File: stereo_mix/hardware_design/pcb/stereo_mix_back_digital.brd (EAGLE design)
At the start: 75 x 100 mm, 233 parts, among them IC1 TL072D, IC10 LD117AS50TR, IC11 MCP4822E-SN, IC12 MCP4822E-SN, IC13 MCP4822E-SN, IC14 MCP4822E-SN, IC15 TL072D, IC16 TL072D, IC17 TL072D, IC18 TL072D, IC2 TL072D, IC3 TL072D, IC4 TL072D, IC5 TL072D, IC6 TL072D, IC7 TL072D, IC8 TL072D, IC9 TL072D, Q1 20MHz, U1 MCP6002_, U10 MCP6002_, U11 MCP4922, U12 MCP4922, U13 ATMEGA328P-AU, U14 TEXAS_INSTRUMENTS_LM4040C5IDB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, U15 TEXAS_INSTRUMENTS_LM4040C10ID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, U16 TEXAS_INSTRUMENTS_LM4040C10ID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, U2 MCP6002_, U3 MCP6002_, U4 MCP6002_, U5 MCP4922, U6 MCP4922, U7 MCP6002_, U8 MCP6002_, U9 MCP6002_

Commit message: Add new revision of stereo_mix_back hardware, and associated assembly files
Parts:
- removed IC10: LD117AS50TR, v-reg:SOT223
- removed IC11, IC12, IC13, IC14: MCP4822E-SN, dac:SOIC-8
- removed IC15, IC16, IC17, IC18, IC2, IC3, IC4, IC5, IC6, IC7, IC8, IC9: TL072D, linear:SO08
- added D3: LM4040AIM3-5.0, jhbruhn-ref:SOT23
- added D4, D5: LM4040AIM3-10.0, jhbruhn-ref:SOT23
- added U17, U18, U21, U22, U26, U27, U28, U29, U30: TL072AD, jhbruhn-opamp:SOIC8
- added U19, U20, U24, U25: MCP4822E-SN, jhbruhn-dac:SOIC8
- added U23: ATMEGA328P-AU, jhbruhn-mcu:TQFP-32
- C1, C10, C13, C14, C15, C16, C17, C18, C2, C21, C22, C23, C24, C27, C28, C29, C3, C30, C31, C32, C36, C37, C38, C4, C47, C5, C50, C51, C52, C53, C54, C58, C6, C61, C62, C63, C7, C8, C9: device resistor:C0402 -> jhbruhn-cr:C0402
- C11, C12, C19, C20: value 100nF -> 4.7nF; device resistor:C0402 -> jhbruhn-cr:C0402
- C25, C26: value 18pF -> 100nF; device resistor:C0402 -> jhbruhn-cr:C0402
- C33: value EURO_POWER_LOCKFAT-LOCK -> 100nF; device MusicThingModular:EURO_PWR_HEADER_LOCK -> jhbruhn-cr:C0402
- C34, C35, C45, C46: value 47uF -> 100nF; device rcl:PANASONIC_C -> jhbruhn-cr:C0402
- C39, C40, C41, C42: value 4.7nF -> 100nF; device resistor:C0402 -> jhbruhn-cr:C0402
- C43, C44: value 6.8pF -> 18pF; device resistor:C0402 -> jhbruhn-cr:C0402
- C48, C49: value 100nF -> 6.8pF; device resistor:C0402 -> jhbruhn-cr:C0402
- C55: value 100nF -> EURO_POWER_LOCKFAT-LOCK; device resistor:C0402 -> MusicThingModular:EURO_PWR_HEADER_LOCK
- C56, C57, C59, C60: value 100nF -> 47uF; device resistor:C0402 -> rcl:PANASONIC_C
- IC1: value TL072D -> LD117AS50TR; device linear:SO08 -> v-reg:SOT223
- R1, R10, R105, R11, R110, R111, R112, R113, R114, R115, R12, R13, R14, R15, R16, R17, R18, R19, R2, R20, R21, R22, R23, R24, R25, R26, R27, R28, R29, R3, R30, R31, R32, R33, R34, R35, R36, R37, R38, R39, R4, R40, R41, R42, R43, R44, R45, R46, R47, R48, R49, R5, R50, R51, R52, R53, R54, R55, R56, R57, R58, R59, R6, R60, R61, R62, R63, R64, R65, R66, R67, R68, R69, R7, R70, R71, R72, R73, R74, R75, R76, R77, R78, R79, R8, R80, R81, R82, R83, R84, R85, R86, R87, R88, R89, R9, R90, R91, R92, R97, R98, R99: device resistor:R0402 -> jhbruhn-cr:R0402
- R100: value 24k -> 100k; device resistor:R0402 -> jhbruhn-cr:R0402
- R101: value 24k -> 43k; device resistor:R0402 -> jhbruhn-cr:R0402
- R102, R103, R104, R94, R95, R96: value 100k -> 43k; device resistor:R0402 -> jhbruhn-cr:R0402
- R106, R107, R108: value 402R -> 100k; device resistor:R0402 -> jhbruhn-cr:R0402
- R109: value 100k -> 10k; device resistor:R0402 -> jhbruhn-cr:R0402
- R116: value 100k -> 24k; device resistor:R0402 -> jhbruhn-cr:R0402
- R117: value 43k -> 24k; device resistor:R0402 -> jhbruhn-cr:R0402
- R118, R119, R120, R121: value 43k -> 100k; device resistor:R0402 -> jhbruhn-cr:R0402
- R122, R123, R124: value 43k -> 470R; device resistor:R0402 -> jhbruhn-cr:R0402
- R93: value 10k -> 43k; device resistor:R0402 -> jhbruhn-cr:R0402
- U1, U10, U8, U9: value MCP6002_ -> TL072AD; device MusicThingModular:SO08 -> jhbruhn-opamp:SOIC8
- U11, U12, U5: value MCP4922 -> MCP6002E/SN; device MCP4922:SO-14 -> jhbruhn-opamp:SOIC8
- U13: value ATMEGA328P-AU -> MCP6002E/SN; device Microcontroller:TQFP-32 -> jhbruhn-opamp:SOIC8
- U14: value TEXAS_INSTRUMENTS_LM4040C5IDBZR -> MCP6002E/SN; device lm4040:TEXAS_INSTRUMENTS_LM4040C5IDBZR_0 -> jhbruhn-opamp:SOIC8
- U15, U16: value TEXAS_INSTRUMENTS_LM4040C10IDBZR -> MCP4922E/SL; device lm4040:TEXAS_INSTRUMENTS_LM4040C5IDBZR_0 -> jhbruhn-dac:SO-14
- U2, U3, U4: value MCP6002_ -> MCP6002E/SN; device MusicThingModular:SO08 -> jhbruhn-opamp:SOIC8
- U6: value MCP4922 -> MCP4922E/SL; device MCP4922:SO-14 -> jhbruhn-dac:SO-14
- U7: value MCP6002_ -> MCP4922E/SL; device MusicThingModular:SO08 -> jhbruhn-dac:SO-14
- moved C52 195.3 mm to (7.62, 74.3), flipped to the bottom
- moved C63 190.9 mm to (39.4, 1.91), flipped to the bottom, turned to 180 degrees
- moved C57 190.4 mm to (14.0, 41.9), flipped to the bottom
- moved C53 189.8 mm to (7.62, 63.5), flipped to the bottom
- moved C56 188.0 mm to (21.6, 41.9), flipped to the bottom, turned to 180 degrees
- moved C62 187.7 mm to (8.89, 15.2), flipped to the bottom, turned to 180 degrees
- moved C54 184.9 mm to (7.62, 53.3), flipped to the bottom
- moved C61 184.7 mm to (45.7, 1.91), flipped to the bottom
- moved C60 180.6 mm to (5.08, 19.1), flipped to the bottom, turned to 180 degrees
- moved C55 177.8 mm to (3.81, 41.9), flipped to the bottom, turned to 90 degrees
- moved C58 174.9 mm to (52.1, 1.91), flipped to the bottom
- moved C59 161.1 mm to (5.08, 3.81), flipped to the bottom
- moved R120 158.2 mm to (7.62, 61.0), flipped to the bottom, turned to 180 degrees
- moved R121 153.4 mm to (7.62, 50.8), flipped to the bottom, turned to 180 degrees
- moved R118 149.8 mm to (7.62, 62.2), flipped to the bottom
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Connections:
- removed net 3_CV_PAN_IN: R43.1, R44.1
- removed net N$84: C52.1, C53.1, C54.1, C55.1, IC11.1, IC12.1, IC13.1, IC14.1
- removed net N$85: C52.2, C53.2, C55.2, IC11.7, IC12.7, IC13.7, IC14.7
- net +12V: now also C13.1, C41.1, C42.1, C45.1, C46.1, C52.1, C53.1, C54.1, C56.+, C59.+, IC1.3, R122.2, R123.2, U1.8, U10.8, U17.8, U18.8, U21.8, U22.8, U26.8, U27.8, U28.8, U29.8, U30.8, U8.8, U9.8; no longer C11.1, C30.1, C31.1, C32.1, C34.+, C45.+, C60.1, C61.1, C62.1, C63.1, IC1.8, IC10.3, IC15.8, IC16.8, IC17.8, IC18.8, IC2.8, IC3.8, IC4.8, IC5.8, IC6.8, IC7.8, IC8.8, IC9.8, R106.2, R107.2
- net +5V: now also C24.1, C25.1, C26.1, C27.1, C28.1, C29.1, C30.1, C31.1, C32.1, C33.1, C35.1, C36.1, C60.+, C62.1, IC1.4, R109.2, U11.8, U12.8, U13.8, U14.8, U15.1, U15.9, U16.1, U16.9, U19.1, U20.1, U23.18, U23.4, U23.6, U24.1, U25.1, U5.8, U7.1, U7.9; no longer C13.1, C14.1, C19.1, C20.1, C46.+, C47.1, C48.1, C49.1, C50.1, C51.1, IC10.4, R93.2, U1.8, U10.8, U11.1, U11.9, U12.1, U12.9, U13.18, U13.4, U13.6, U5.1, U5.9, U7.8, U8.8, U9.8
- net -12V: now also C14.2, C37.2, C38.2, C39.2, C40.2, C47.2, C50.2, C51.2, C57.-, R124.2, U1.4, U10.4, U17.4, U18.4, U21.4, U22.4, U26.4, U27.4, U28.4, U29.4, U30.4, U8.4, U9.4; no longer C12.2, C27.2, C28.2, C29.2, C35.-, C56.2, C57.2, C58.2, C59.2, IC1.4, IC15.4, IC16.4, IC17.4, IC18.4, IC2.4, IC3.4, IC4.4, IC5.4, IC6.4, IC7.4, IC8.4, IC9.4, R108.2
- net 1_PAN_ATT_W: now also U1.3; no longer IC1.3
- net 2_PAN_ATT_W: now also U1.5; no longer IC1.5
- net 3_PAN_ATT_W: now also U10.3; no longer IC4.3
- net 3_PAN_CV_IN: now also R43.1, R44.1
- net 4_PAN_ATT_W: now also U10.5; no longer IC4.5
- net AREF_-10: now also C63.1, D5.2, R124.1; no longer C38.1, R108.1, U16.2
- net AUX_IN_L: now also R110.1; no longer R94.1
- net AUX_IN_R: now also R111.1; no longer R95.1
- net BAL_N_L: now also R120.2, U29.7; no longer IC8.7, R104.2
- net BAL_N_R: now also R121.2, U30.7; no longer IC9.7, R105.2
- net BAL_P_L: now also R116.2, R118.1, U29.1; no longer IC8.1, R100.2, R102.1
- net BAL_P_R: now also R117.2, R119.1, U30.1; no longer IC9.1, R101.2, R103.1
- net BIAS_DAC1_L: now also R97.2, U21.1; no longer IC15.1, R109.2
- net BIAS_DAC1_R: now also R98.2, U21.7; no longer IC15.7, R110.2
- net BIAS_DAC2_L: now also R99.2, U22.1; no longer IC16.1, R111.2
- net BIAS_DAC2_R: now also R100.2, U22.7; no longer IC16.7, R112.2
- net BIAS_DAC3_L: now also R105.2, U26.1; no longer IC17.1, R113.2
- net BIAS_DAC3_R: now also R106.2, U26.7; no longer IC17.7, R114.2
- net BIAS_DAC4_L: now also R107.2, U27.1; no longer IC18.1, R115.2
- net BIAS_DAC4_R: now also R108.2, U27.7; no longer IC18.7, R116.2
- net BYPASS_L: now also C48.2, R112.2, U28.1; no longer C43.2, IC7.1, R96.2
- net BYPASS_R: now also C49.2, R113.2, U28.7; no longer C44.2, IC7.7, R97.2
- net CS_BIAS_DAC_1: now also U19.2, U23.2; no longer IC11.2, U13.2
- net CS_BIAS_DAC_2: now also U20.2, U23.9; no longer IC12.2, U13.9
- net CS_BIAS_DAC_3: now also U23.10, U24.2; no longer IC13.2, U13.10
- net CS_BIAS_DAC_4: now also U23.11, U25.2; no longer IC14.2, U13.11
- net CS_DAC_1: now also U23.30, U6.3; no longer U13.30, U5.3
- net CS_DAC_2: now also U23.31, U7.3; no longer U13.31, U6.3
- net CS_DAC_3: now also U15.3, U23.32; no longer U11.3, U13.32
- net CS_DAC_4: now also U16.3, U23.1; no longer U12.3, U13.1
- net GND: now also C14.1, C27.2, C28.2, C29.2, C33.2, C34.2, C35.2, C37.1, C38.1, C39.1, C40.1, C41.2, C42.2, C43.2, C44.2, C45.2, C46.2, C47.1, C50.1, C51.1, C52.2, C53.2, C54.2, C55.GND1, C55.GND2, C55.GND3, C55.GND4, C55.GND5, C55.GND6, C56.-, C57.+, C58.2, C59.-, C60.-, D3.2, D4.2, D5.1, IC1.1, U11.3, U11.4, U11.5, U12.3, U12.4, U12.5, U13.4, U14.3, U14.4, U14.5, U15.12, U15.8, U16.12, U16.8, U17.3, U17.5, U18.3, U18.5, U19.5, U19.7, U20.5, U20.7, U21.3, U21.5, U22.3, U22.5, U23.21, U23.3, U23.5, U24.5, U24.7, U25.5, U25.7, U26.3, U26.5, U27.3, U27.5, U28.3, U28.5, U29.3, U29.5, U30.3, U30.5, U4.3, U4.5, U5.4, U7.12, U7.8, U9.3, U9.5; no longer C11.2, C12.1, C14.2, C19.2, C20.2, C27.1, C28.1, C29.1, C33.GND1, C33.GND2, C33.GND3, C33.GND4, C33.GND5, C33.GND6, C34.-, C35.+, C37.2, C38.2, C45.-, C46.-, C47.2, C48.2, C49.2, C50.2, C51.2, C56.1, C57.1, C58.1, C59.1, C60.2, IC10.1, IC11.5, IC12.5, IC13.5, IC14.5, IC15.3, IC15.5, IC16.3, IC16.5, IC17.3, IC17.5, IC18.3, IC18.5, IC2.3, IC2.5, IC3.3, IC3.5, IC5.3, IC5.5, IC6.3, IC6.5, IC7.3, IC7.5, IC8.3, IC8.5, IC9.3, IC9.5, U1.3, U1.4, U1.5, U10.3, U10.4, U10.5, U11.12, U11.8, U12.12, U12.8, U13.21, U13.3, U13.5, U14.2, U15.2, U16.1, U5.12, U5.8, U7.3, U7.4, U7.5, U8.4, U9.4
- net MISO: now also U23.16; no longer U13.16
- net MOSI: now also U15.5, U16.5, U19.4, U20.4, U23.15, U24.4, U25.4, U7.5; no longer IC11.4, IC12.4, IC13.4, IC14.4, U11.5, U12.5, U13.15, U5.5
- net N$1: now also U6.14; no longer U5.14
- net N$10: now also U6.10; no longer U5.10
- net N$11: now also C43.1, U23.8; no longer C25.1, U13.8
- net N$12: now also C11.1, U4.2; no longer C39.1, U3.2
- net N$13: now also U1.1; no longer IC1.1
- net N$14: now also R93.1, U19.8; no longer IC11.8, R117.1
- net N$15: now also U5.3; no longer U4.3
- net N$16: now also R94.1, U19.6; no longer IC11.6, R118.1
- net N$17: now also U5.5; no longer U4.5
- net N$18: now also U1.2; no longer IC1.2
- net N$19: now also U3.6; no longer U2.6
- net N$2: now also U2.6; no longer U1.6
- net N$20: now also U3.7, U7.11; no longer U2.7, U6.11
- net N$21: now also U3.1, U7.13; no longer U2.1, U6.13
- net N$22: now also U3.2; no longer U2.2
- net N$23: now also U7.14; no longer U6.14
- net N$24: now also U9.2; no longer IC3.2
- net N$25: now also U9.1; no longer IC3.1
- net N$26: now also U9.6; no longer IC3.6
- net N$27: now also U7.10; no longer U6.10
- net N$28: now also U9.7; no longer IC3.7
- net N$29: now also U11.6; no longer U7.6
- net N$3: now also U8.2; no longer IC2.2
- net N$30: now also U11.7, U15.11; no longer U11.11, U7.7
- net N$31: now also U11.1, U15.13; no longer U11.13, U7.1
- net N$32: now also R114.1, R116.1, U29.2; no longer IC8.2, R100.1, R98.1
- net N$33: now also U11.2; no longer U7.2
- net N$34: now also U15.14; no longer U11.14
- net N$35: now also U17.2; no longer IC5.2
- net N$36: now also U17.1; no longer IC5.1
- net N$37: now also U17.6; no longer IC5.6
- net N$38: now also U15.10; no longer U11.10
- net N$39: now also U17.7; no longer IC5.7
- net N$4: now also U2.1, U6.13; no longer U1.1, U5.13
- net N$40: now also U12.6; no longer U8.6
- net N$41: now also U12.7, U16.11; no longer U12.11, U8.7
- net N$42: now also C12.1, U4.6; no longer C40.1, U3.6
- net N$43: now also R119.2, R121.1, U30.6; no longer IC9.6, R103.2, R105.1
- net N$44: now also U12.1, U16.13; no longer U12.13, U8.1
- net N$45: now also R118.2, R120.1, U29.6; no longer IC8.6, R102.2, R104.1
- net N$46: now also U12.2; no longer U8.2
- net N$47: now also C55.POS1, C55.POS2; no longer C33.POS1, C33.POS2
- net N$48: now also C55.NEG1, C55.NEG2; no longer C33.NEG1, C33.NEG2
- net N$49: now also U16.14; no longer U12.14
- net N$5: now also U2.7, U6.11; no longer U1.7, U5.11
- net N$50: now also U18.2; no longer IC6.2
- net N$51: now also U18.1; no longer IC6.1
- net N$52: now also U18.6; no longer IC6.6
- net N$53: now also U16.10; no longer U12.10
- net N$54: now also U18.7; no longer IC6.7
- net N$55: now also R115.1, R117.1, U30.2; no longer IC9.2, R101.1, R99.1
- net N$56: now also U1.7; no longer IC1.7
- net N$57: now also U1.6; no longer IC1.6
- net N$58: now also C34.1, U23.20; no longer C24.1, U13.20
- net N$59: now also C19.1, U14.2; no longer C41.1, U10.2
- net N$6: now also U2.2; no longer U1.2
- net N$60: now also U10.1; no longer IC4.1
- net N$61: now also U10.2; no longer IC4.2
- net N$62: now also C44.1, U23.7; no longer C26.1, U13.7
- net N$63: now also C20.1, U14.6; no longer C42.1, U10.6
- net N$64: now also U10.7; no longer IC4.7
- net N$65: now also U10.6; no longer IC4.6
- net N$66: now also U13.3; no longer U9.3
- net N$67: now also R95.1, U20.8; no longer IC12.8, R119.1
- net N$68: now also R96.1, U20.6; no longer IC12.6, R120.1
- net N$69: now also U13.5; no longer U9.5
- net N$7: now also U8.7; no longer IC2.7
- net N$70: now also R101.1, U24.8; no longer IC13.8, R121.1
- net N$71: now also R102.1, U24.6; no longer IC13.6, R122.1
- net N$72: now also R103.1, U25.8; no longer IC14.8, R123.1
- net N$73: now also R104.1, U25.6; no longer IC14.6, R124.1
- net N$74: now also R93.2, R97.1, U21.2; no longer IC15.2, R109.1, R117.2
- net N$75: now also R94.2, R98.1, U21.6; no longer IC15.6, R110.1, R118.2
- net N$76: now also R95.2, R99.1, U22.2; no longer IC16.2, R111.1, R119.2
- net N$77: now also R100.1, R96.2, U22.6; no longer IC16.6, R112.1, R120.2
- net N$78: now also R101.2, R105.1, U26.2; no longer IC17.2, R113.1, R121.2
- net N$79: now also R102.2, R106.1, U26.6; no longer IC17.6, R114.1, R122.2
- net N$8: now also U8.1; no longer IC2.1
- net N$80: now also R103.2, R107.1, U27.2; no longer IC18.2, R115.1, R123.2
- net N$81: now also R104.2, R108.1, U27.6; no longer IC18.6, R116.1, R124.2
- net N$9: now also U8.6; no longer IC2.6
- net OUT_L: now also R114.2; no longer R98.2
- net OUT_R: now also R115.2; no longer R99.2
- net PAN_CV_1: now also C11.2, U23.27, U4.1; no longer C39.2, U13.27, U3.1
- net PAN_CV_2: now also C12.2, U23.28, U4.7; no longer C40.2, U13.28, U3.7
- net PAN_CV_3: now also C19.2, U14.1, U23.19; no longer C41.2, U10.1, U13.19
- net PAN_CV_4: now also C20.2, U14.7, U23.22; no longer C42.2, U10.7, U13.22
- net REF_10: now also C61.1, D4.1, R123.1; no longer C37.1, R107.1, U15.1
- net REF_5: now also C58.1, D3.1, R122.1; no longer C36.1, R106.1, U14.1
- net RESET: now also R109.1, U23.29; no longer R93.1, U13.29
- net SCK: now also U15.4, U16.4, U19.3, U20.3, U23.17, U24.3, U25.3, U7.4; no longer IC11.3, IC12.3, IC13.3, IC14.3, U11.4, U12.4, U13.17, U5.4
- net SUM_L: now also C48.1, R110.2, R112.1, U28.2; no longer C43.1, IC7.2, R94.2, R96.1
- net SUM_R: now also C49.1, R111.2, R113.1, U28.6; no longer C44.1, IC7.6, R95.2, R97.1
- net VOL_CV_1: now also U23.23, U5.1, U5.2; no longer U13.23, U4.1, U4.2
- net VOL_CV_2: now also U23.24, U5.6, U5.7; no longer U13.24, U4.6, U4.7
- net VOL_CV_3: now also U13.1, U13.2, U23.25; no longer U13.25, U9.1, U9.2
- net VOL_CV_4: now also U13.6, U13.7, U23.26; no longer U13.26, U9.6, U9.7
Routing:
- net GND: track 858.4 -> 1101.3 mm, vias 35 -> 111
- net CS_BIAS_DAC_2: track 0.00 -> 173.2 mm, vias 0 -> 6
- net +12V: track 315.1 -> 479.8 mm, vias 16 -> 15
- net AREF_-10: track 364.1 -> 201.1 mm, vias 25 -> 20
- net CS_BIAS_DAC_1: track 0.00 -> 136.2 mm, vias 0 -> 6
- net -12V: track 266.7 -> 392.2 mm, vias 17 -> 20
- net +5V: track 342.7 -> 448.8 mm, vias 24 -> 21
- net CS_BIAS_DAC_3: track 0.00 -> 103.4 mm, vias 0 -> 8
- net MOSI: track 127.3 -> 206.3 mm, vias 8 -> 1
- net CS_BIAS_DAC_4: track 0.00 -> 73.7 mm, vias 0 -> 8
- net BIAS_DAC4_R: track 0.00 -> 63.5 mm, vias 0 -> 6
- net REF_10: track 37.8 -> 100.4 mm, vias 4 -> 5
- net BAL_N_R: track 81.3 -> 139.1 mm, vias 2 -> 7
- net SCK: track 141.8 -> 199.5 mm
- net SUM_R: track 143.7 -> 92.3 mm, vias 6 -> 0
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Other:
- board text added: "dont break this"
- board text added: "jhbruhn 2019 stereo mix back digital v1.1"
- board text added: "not so low, ruediger!"
- board text added: "plsgovegan"
- board text removed: "jhbruhn 2019 stereo mix back digital"

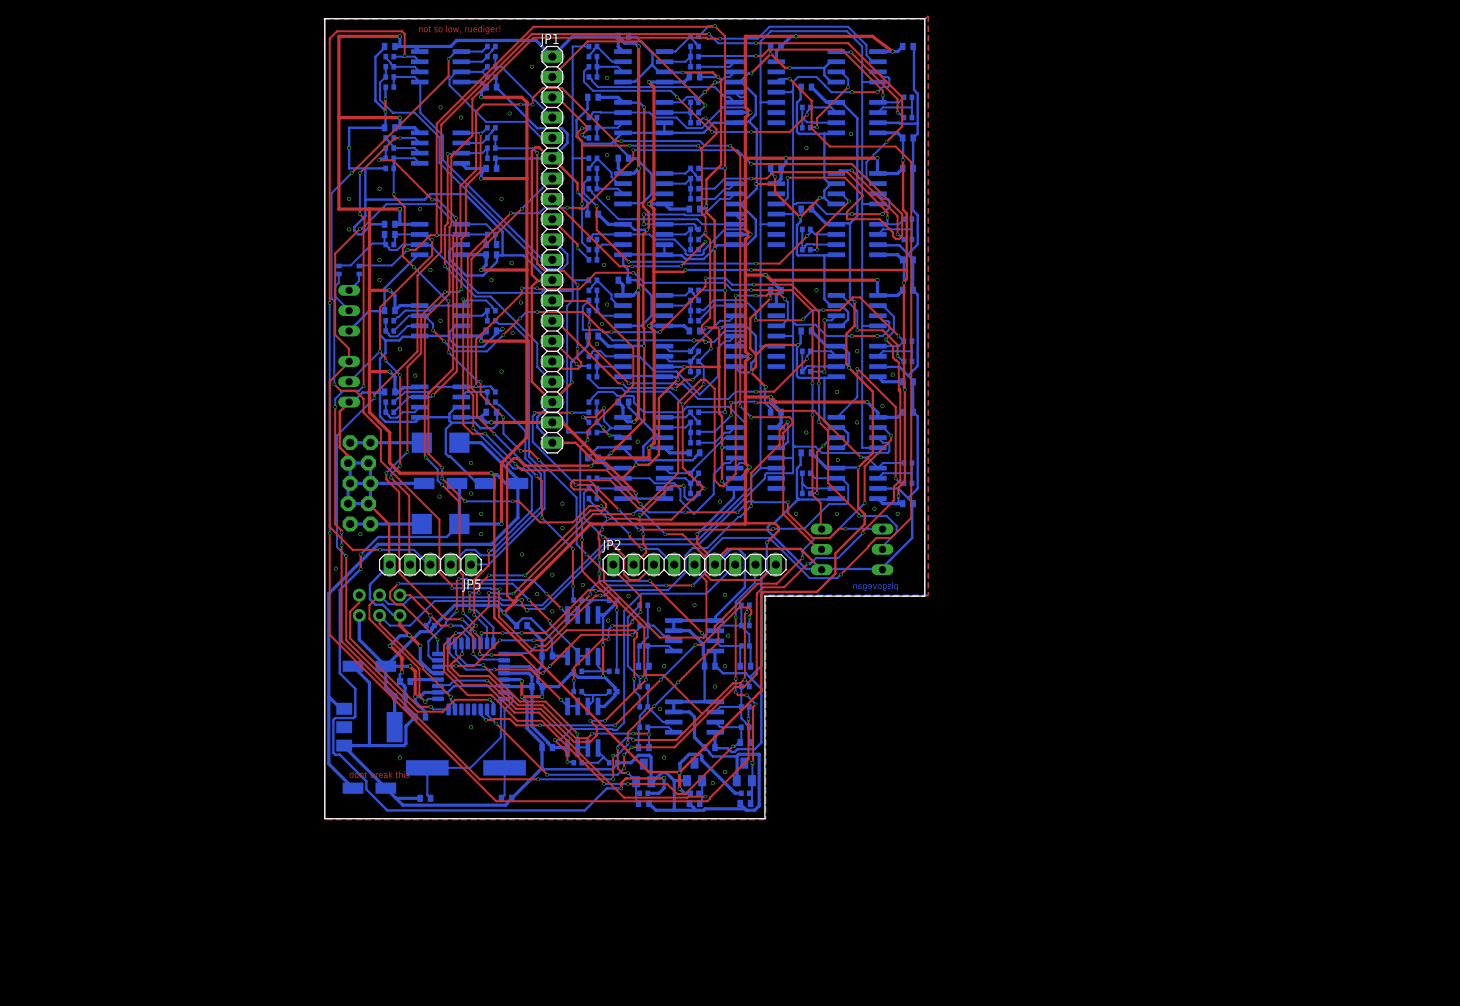
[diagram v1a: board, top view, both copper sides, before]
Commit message: Start revamp of stereo mix pcb
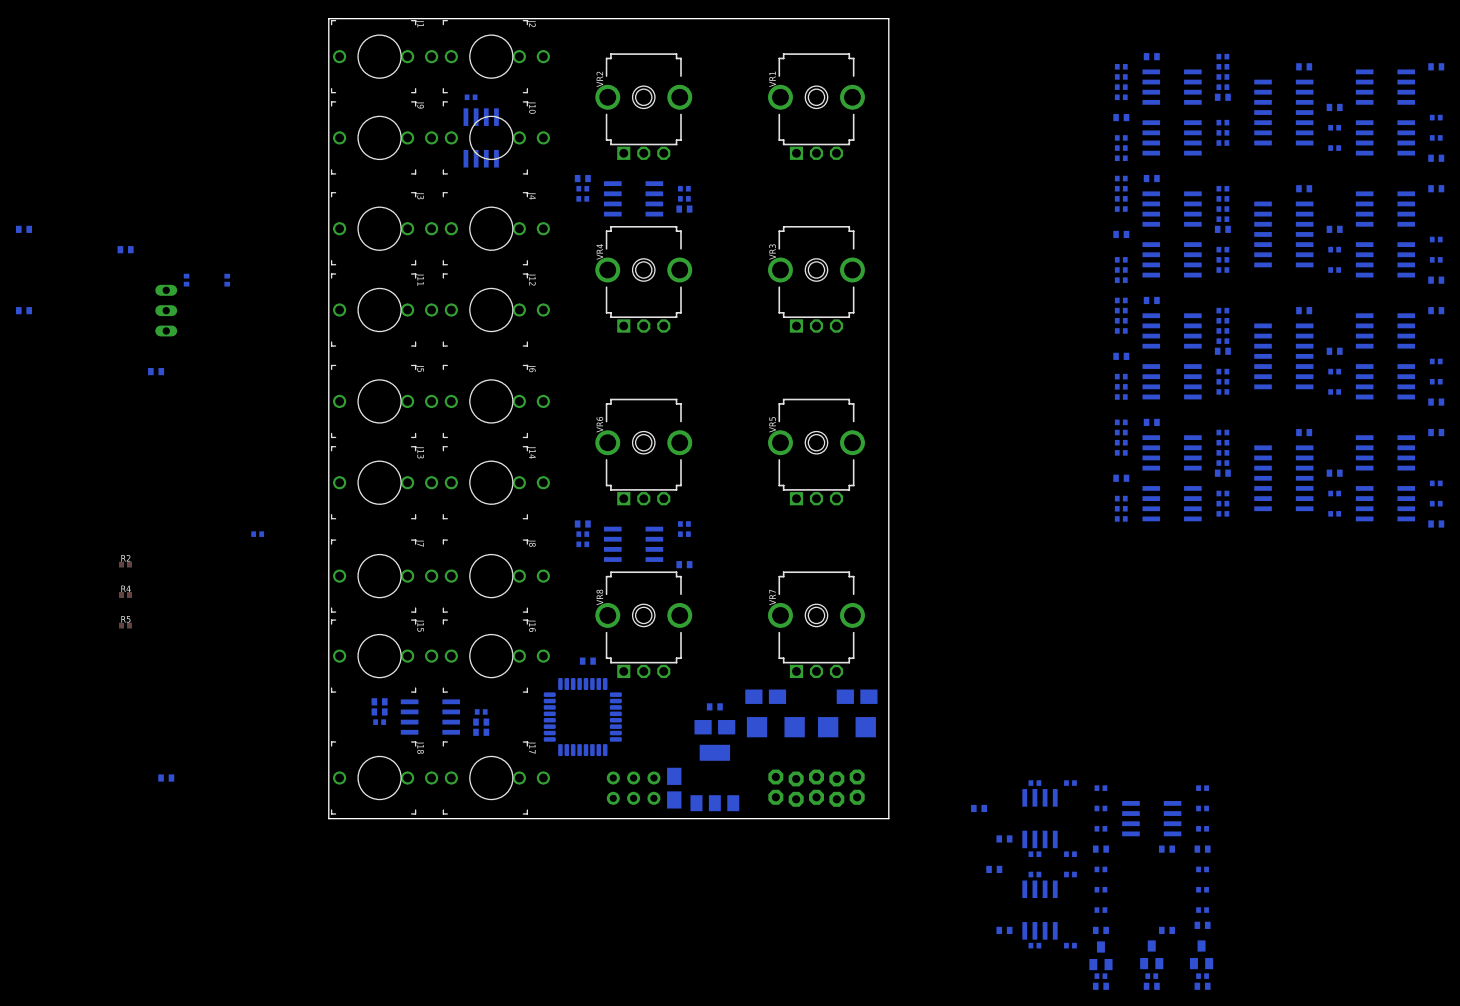
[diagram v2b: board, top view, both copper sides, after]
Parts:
- removed C43, C44: 18pF, jhbruhn-cr:C0402
- removed JP1: (no value), pinhead:1X20
- removed JP2: (no value), pinhead:1X09
- removed JP4, JP6, JP7: (no value), jumper:JP2
- removed JP5: (no value), pinhead:1X05
- removed Q1: 20MHz, crystal:HC49UP
- removed R115, R118, R119, R120, R121, R44, R46, R49, R50, R6: 100k, jhbruhn-cr:R0402
- removed R116, R117: 24k, jhbruhn-cr:R0402
- removed U29, U30: TL072AD, jhbruhn-opamp:SOIC8
- added J1, J10, J11, J12, J13, J14, J15, J16, J17, J18, J2, J3, J4, J5, J6, J7, J8, J9: WQP-PJ301M-12_JACK, jhbruhn-physical:WQP-PJ301M-12_JACK
- added VR1, VR2, VR3, VR4, VR5, VR6, VR7, VR8: (no value), jhbruhn-physical:9MM_SNAP-IN_POT
- C56, C57, C59, C60: device rcl:PANASONIC_C -> rcl:A/3216-18W
- moved R5 82.4 mm to (-25.4, 24.1), flipped to the top
- moved R2 77.2 mm to (-25.4, 31.8), flipped to the top
- moved U4 77.1 mm to (19.1, 85.1), turned to 180 degrees
- moved R4 72.7 mm to (-25.4, 27.9), flipped to the top, turned to 0 degrees
- moved C55 68.7 mm to (61.0, 3.81), turned to 0 degrees
- moved C1 66.1 mm to (102.9, 95.2)
- moved C10 66.1 mm to (111.8, 73.7)
- moved C14 66.1 mm to (111.8, 90.2)
- moved C29 66.1 mm to (138.4, 48.3)
- moved C3 66.1 mm to (102.9, 80.0)
- moved C30 66.1 mm to (138.4, 63.5)
- moved C35 66.1 mm to (138.4, 94.0)
- moved C36 66.1 mm to (138.4, 78.7)
- moved C37 66.1 mm to (138.4, 36.8)
- moved C38 66.1 mm to (138.4, 52.1)
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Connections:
- removed net 1_PAN_ATT_W: JP1.5, R2.2, R5.2, U1.3
- removed net 2_PAN_ATT_W: JP1.11, R4.2, R6.2, U1.5
- removed net 3_PAN_ATT_W: JP1.17, R44.2, R49.2, U10.3
- removed net 4_PAN_ATT_W: JP2.5, R46.2, R50.2, U10.5
- removed net BAL_N_L: JP6.2, R120.2, U29.7
- removed net BAL_N_R: JP7.2, R121.2, U30.7
- removed net BAL_P_L: JP6.1, R116.2, R118.1, U29.1
- removed net BAL_P_R: JP7.1, R117.2, R119.1, U30.1
- removed net BYPASS_L: C48.2, JP4.1, JP5.3, R112.2, U28.1
- removed net BYPASS_R: C49.2, JP4.2, JP5.4, R113.2, U28.7
- removed net N$42: C12.1, R23.2, R24.2, R27.1, U4.6
- removed net N$62: C44.1, Q1.1, U23.7
- removed net N$63: C20.1, R71.2, R72.2, R74.1, U14.6
- new net N$83: U10.3, VR6.2
- net +12V: no longer JP1.1, U29.8, U30.8
- net -12V: no longer JP1.19, U29.4, U30.4
- net 1_IN_L: now also J1.P$1_TIP; no longer JP1.2
- net 1_IN_R: now also J2.P$1_TIP; no longer JP1.3
- net 1_PAN_CV_IN: now also J10.P$1_TIP, R114.1; no longer JP1.4, R1.1, R2.1
- net 1_VOLUME_CV: now also J9.P$1_TIP; no longer JP1.7
- net 2_IN_L: now also J3.P$1_TIP; no longer JP1.8
- net 2_IN_R: now also J4.P$1_TIP; no longer JP1.9
- net 2_PAN_CV_IN: now also J12.P$1_TIP, R2.1; no longer JP1.10, R3.1, R4.1
- net 2_VOLUME_CV: now also J11.P$1_TIP; no longer JP1.13
- net 3_IN_L: now also J5.P$1_TIP; no longer JP1.14
- net 3_IN_R: now also J6.P$1_TIP; no longer JP1.15
- net 3_PAN_CV_IN: now also J14.P$1_TIP, R4.1; no longer JP1.16, R43.1, R44.1
- net 3_VOLUME_CV: now also J13.P$1_TIP; no longer JP2.1
- net 4_IN_L: now also J7.P$1_TIP; no longer JP2.2
- net 4_IN_R: now also J8.P$1_TIP; no longer JP2.3
- net 4_PAN_CV_IN: now also J16.P$1_TIP, R5.1; no longer JP2.4, R45.1, R46.1
- net 4_VOLUME_CV: now also J15.P$1_TIP; no longer JP2.7
- net GND: now also U13.3, U5.3, VR2.1, VR4.1, VR6.1, VR8.1; no longer C43.2, C44.2, JP1.12, JP1.18, JP1.20, JP1.6, JP2.6, JP4.3, JP5.5, JP6.3, JP7.3, R49.1, R5.1, R50.1, R6.1, U14.5, U29.3, U29.5, U30.3, U30.5, U4.5
- net N$11: now also C12.1, R2.2, R23.2, R24.2, R27.1, U5.2; no longer C43.1, Q1.2, U23.8
- net N$12: now also U1.3, VR2.2; no longer C11.1, R21.2, R22.2, R26.1, U4.2
- net N$15: now also U4.5; no longer U5.3
- net N$32: now also C11.1, R114.2, R21.2, R22.2, R26.1, U4.2; no longer R114.1, R116.1, U29.2
- net N$43: now also U1.5, VR4.2; no longer R119.2, R121.1, U30.6
- net N$45: now also U10.5, VR8.2; no longer R118.2, R120.1, U29.6
- net N$55: now also C20.1, R5.2, R71.2, R72.2, R74.1, U13.2; no longer R115.1, R117.1, U30.2
- net N$59: now also R4.2
- net N$66: now also U14.5; no longer U13.3
- net OUT_L: now also C48.2, J17.P$1_TIP, R112.2, U28.1; no longer JP5.1, R114.2
- net OUT_R: now also C49.2, J18.P$1_TIP, R113.2, U28.7; no longer JP5.2, R115.2
- net PAN_CV_2: now also U5.1; no longer U4.7
- net PAN_CV_4: now also U13.1; no longer U14.7
- net REF_10: no longer JP2.9
- net REF_5: now also R1.1, R3.1, R43.1, R45.1, VR2.3, VR4.3, VR6.3, VR8.3; no longer JP2.8
- net VOL_CV_1: now also U4.6, U4.7; no longer U5.1, U5.2
- net VOL_CV_3: now also U14.6, U14.7; no longer U13.1, U13.2
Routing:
- net GND: track 1101.3 -> 0.00 mm, vias 111 -> 0
- net +12V: track 479.8 -> 0.00 mm, vias 15 -> 0
- net +5V: track 448.8 -> 0.00 mm, vias 21 -> 0
- net -12V: track 392.2 -> 0.00 mm, vias 20 -> 0
- net MOSI: track 206.3 -> 0.00 mm, vias 1 -> 0
- net AREF_-10: track 201.1 -> 0.00 mm, vias 20 -> 0
- net SCK: track 199.5 -> 0.00 mm, vias 9 -> 0
- net CS_BIAS_DAC_2: track 173.2 -> 0.00 mm, vias 6 -> 0
- net N$56: track 160.6 -> 0.00 mm, vias 4 -> 0
- net CS_DAC_2: track 149.6 -> 0.00 mm, vias 8 -> 0
- net N$64: track 145.2 -> 0.00 mm, vias 14 -> 0
- net BAL_N_R: track 139.1 -> 0.00 mm, vias 7 -> 0
- net CS_BIAS_DAC_1: track 136.2 -> 0.00 mm, vias 6 -> 0
- net CS_DAC_1: track 134.5 -> 0.00 mm, vias 8 -> 0
- net SUM_L: track 134.0 -> 0.00 mm, vias 6 -> 0
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- removed copper zone on layer 1, net GND
- removed copper zone on layer 16, net GND
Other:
- board size 75 x 100 mm -> 70 x 100 mm
- board text removed: "dont break this"
- board text removed: "not so low, ruediger!"
- board text removed: "plsgovegan"
